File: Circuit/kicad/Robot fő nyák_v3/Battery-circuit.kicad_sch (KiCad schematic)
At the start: 2 parts, among them J1 XT60-M, Q26 IRLHM630PbF

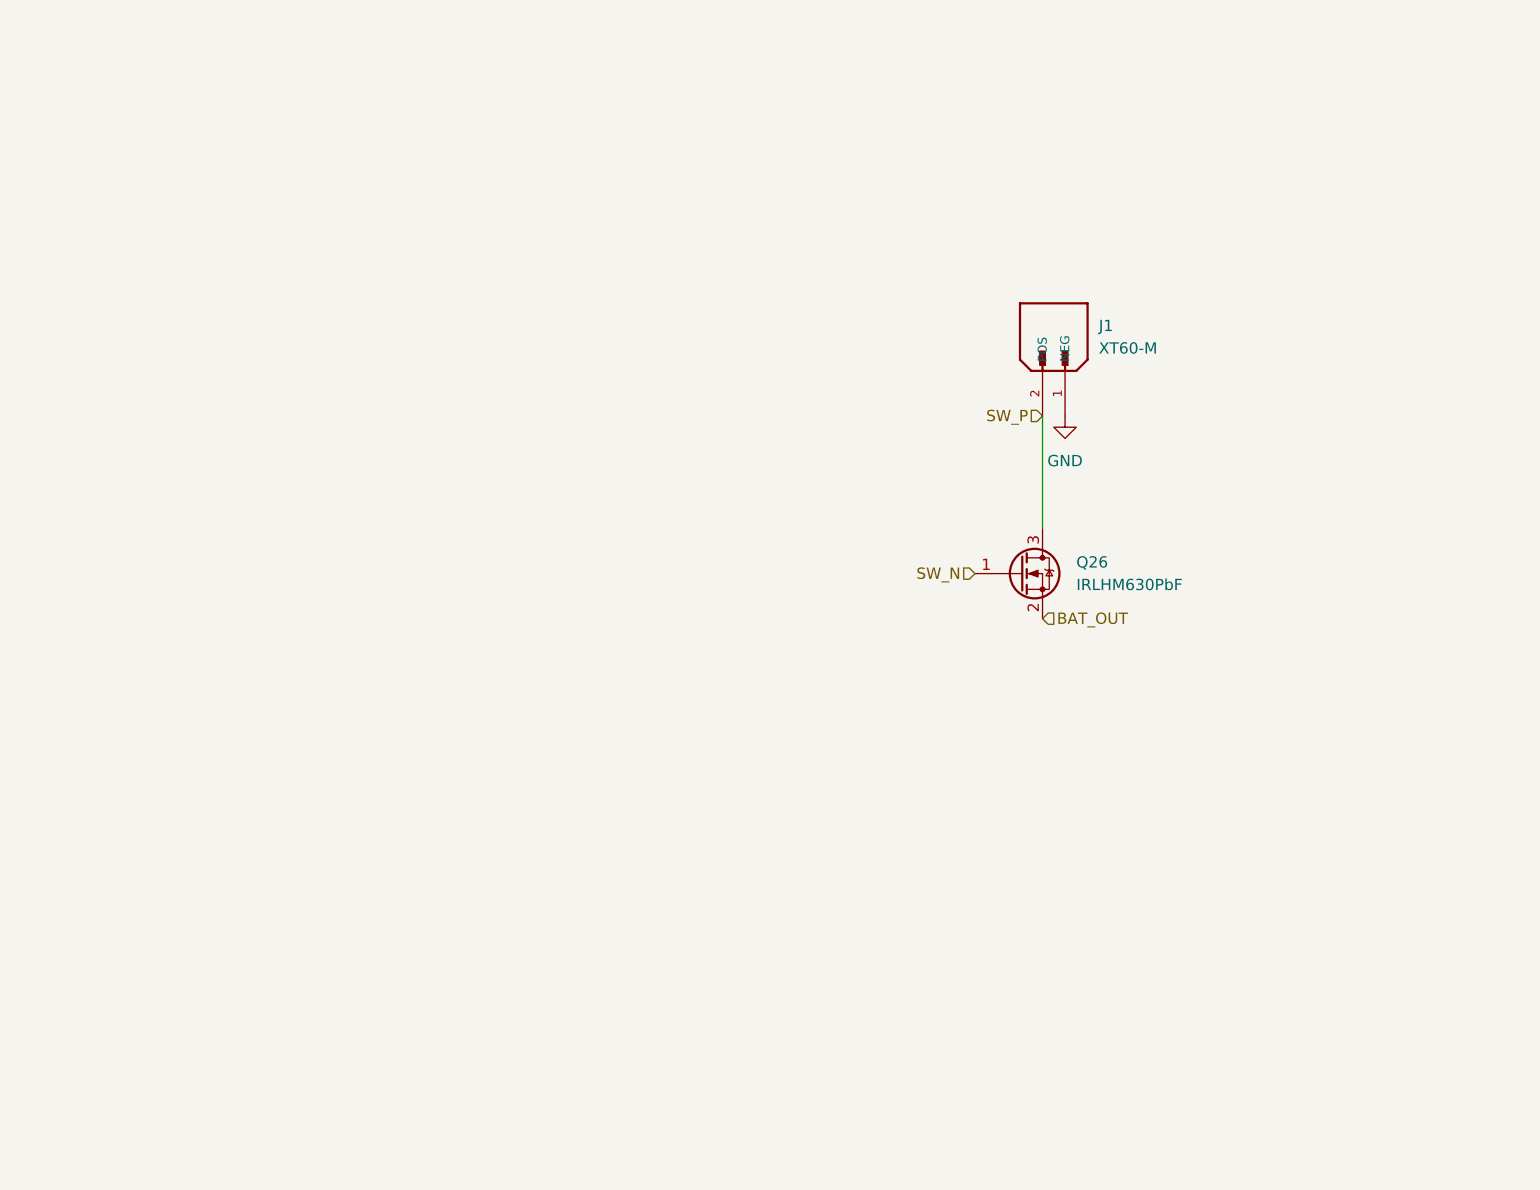
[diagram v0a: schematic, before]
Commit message: kicad update
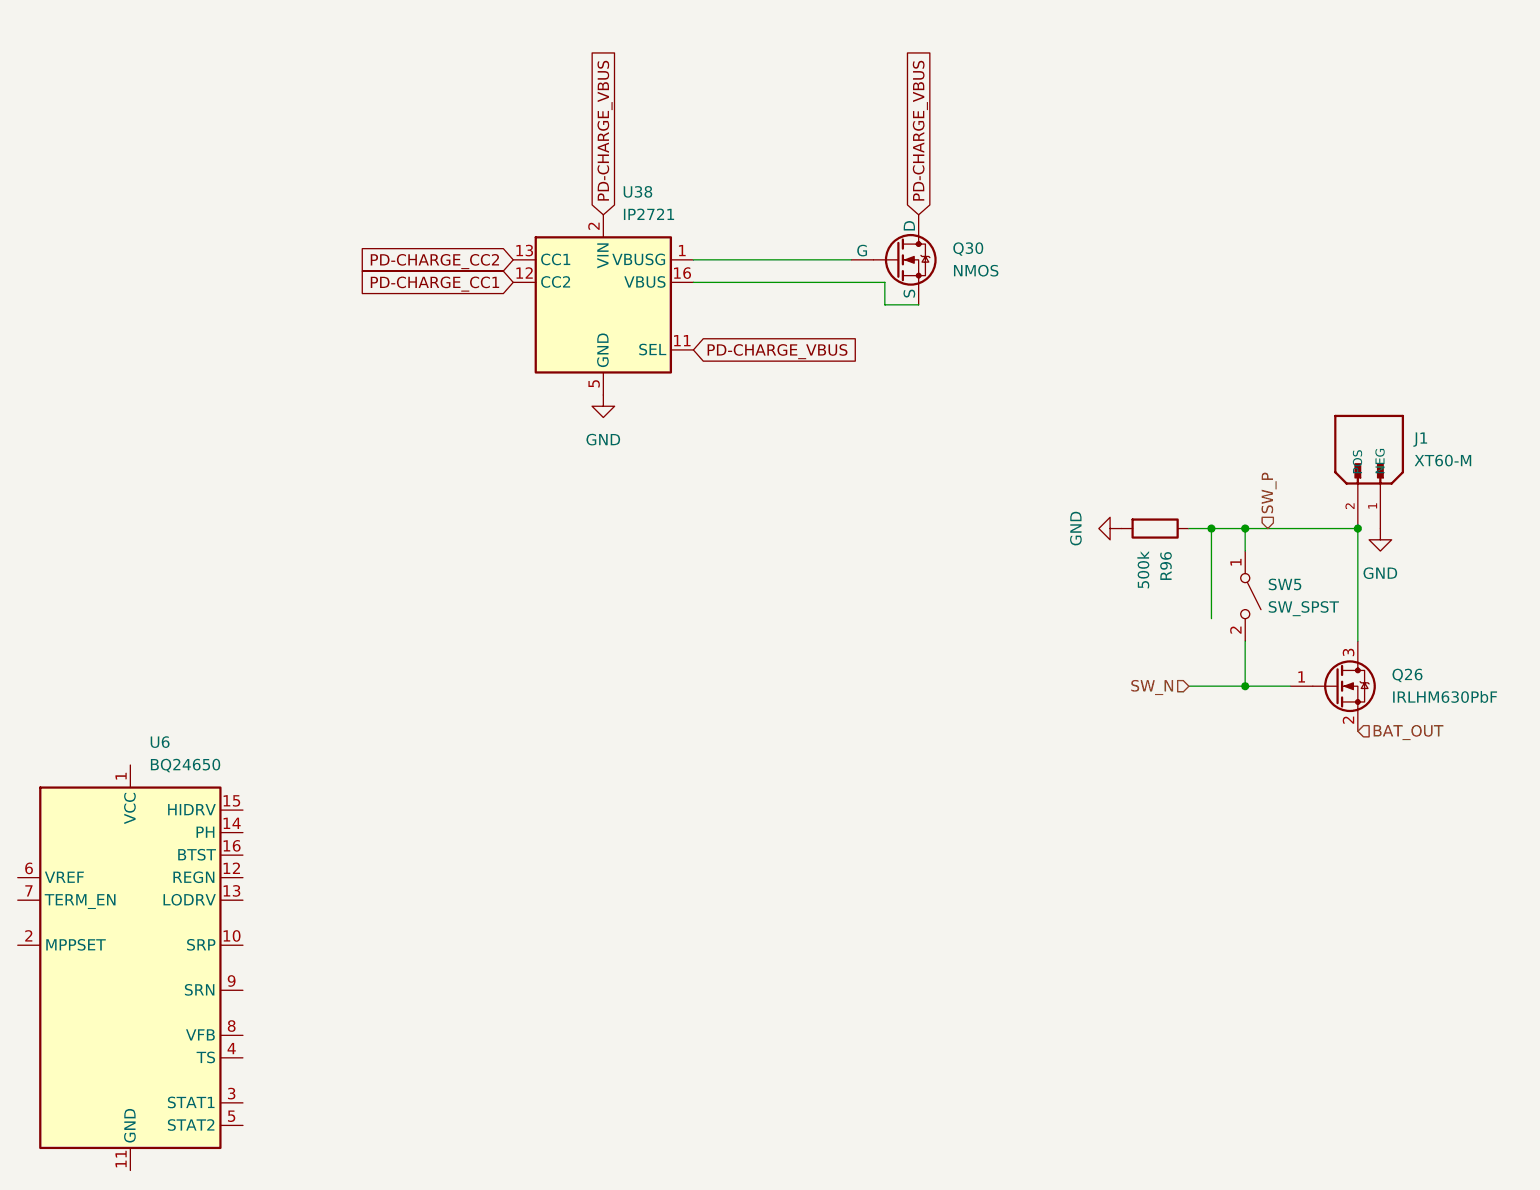
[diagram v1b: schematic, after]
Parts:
- added Q30: NMOS, symbol Simulation_SPICE:NMOS
- added R96: 500k, symbol Device:R
- added SW5: SW_SPST, symbol Switch:SW_SPST
- added U38: IP2721, Package_SO:TSSOP-16_4.4x5mm_P0.65mm, symbol Interface_USB:IP2721
- added U6: BQ24650, Package_DFN_QFN:Texas_RVA_VQFN-16-1EP_3.5x3.5mm_P0.5mm_EP2.14x2.14mm_ThermalVias, symbol Battery_Management:BQ24650
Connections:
- net GND: now also R96.2, U38.5 (GND)
- net SW_N: now also SW5.2 (B)
- net SW_P: now also R96.1, SW5.1 (A)
- new net: Q30.2 (G), U38.1 (VBUSG)
- new net: Q30.3 (S), U38.16 (VBUS)
- new net: U6.11 (GND), U6.17 (GND)
- new net PD-CHARGE_CC1: U38.12 (CC2)
- new net PD-CHARGE_CC2: U38.13 (CC1)
- new net PD-CHARGE_VBUS: Q30.1 (D), U38.11 (SEL), U38.2 (VIN)
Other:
- moved on the sheet: J1, Q26
